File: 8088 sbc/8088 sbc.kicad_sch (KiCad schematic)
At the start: 15 parts, among them U1 8088, U2 74HC573, U3 74HC573, U4 28C256, U5 74HCT00, U6 HM628512, U7 74LS08

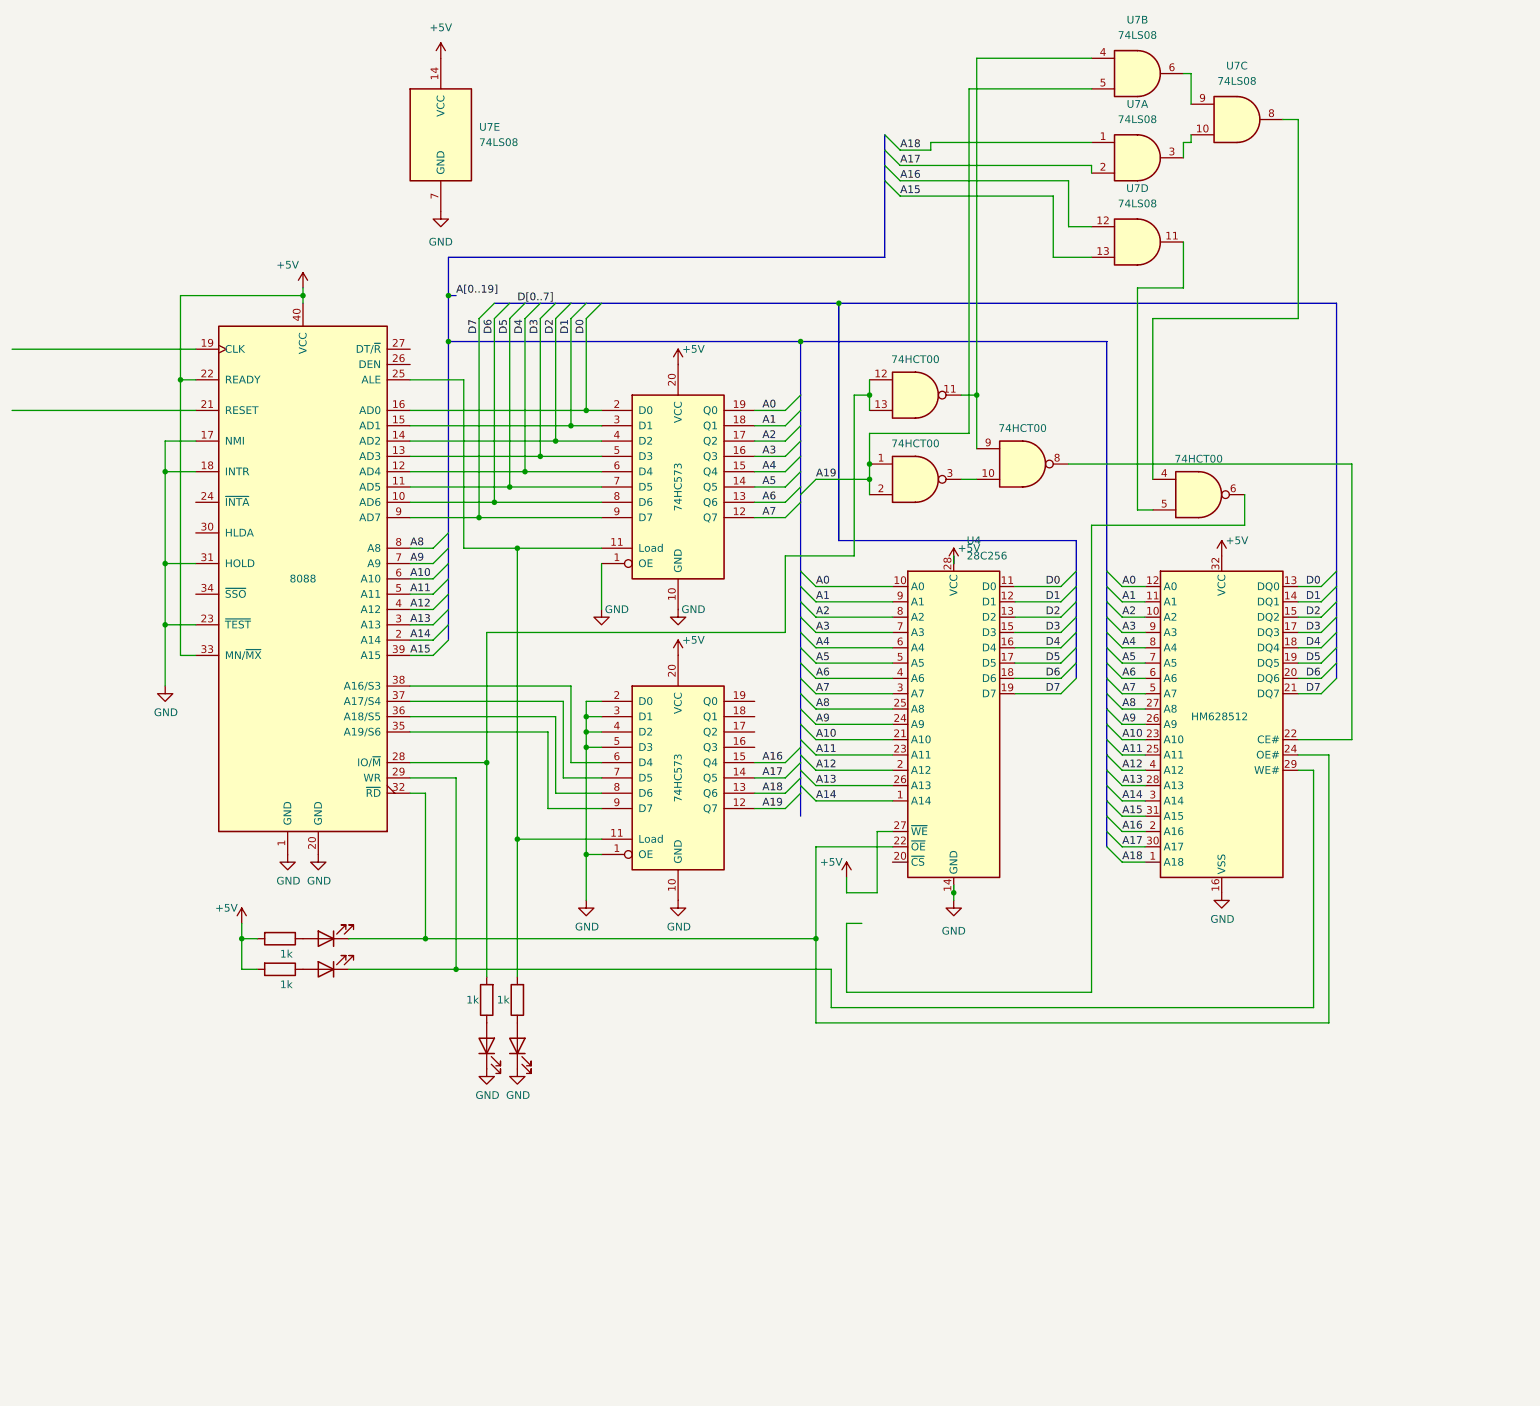
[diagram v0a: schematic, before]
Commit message: e
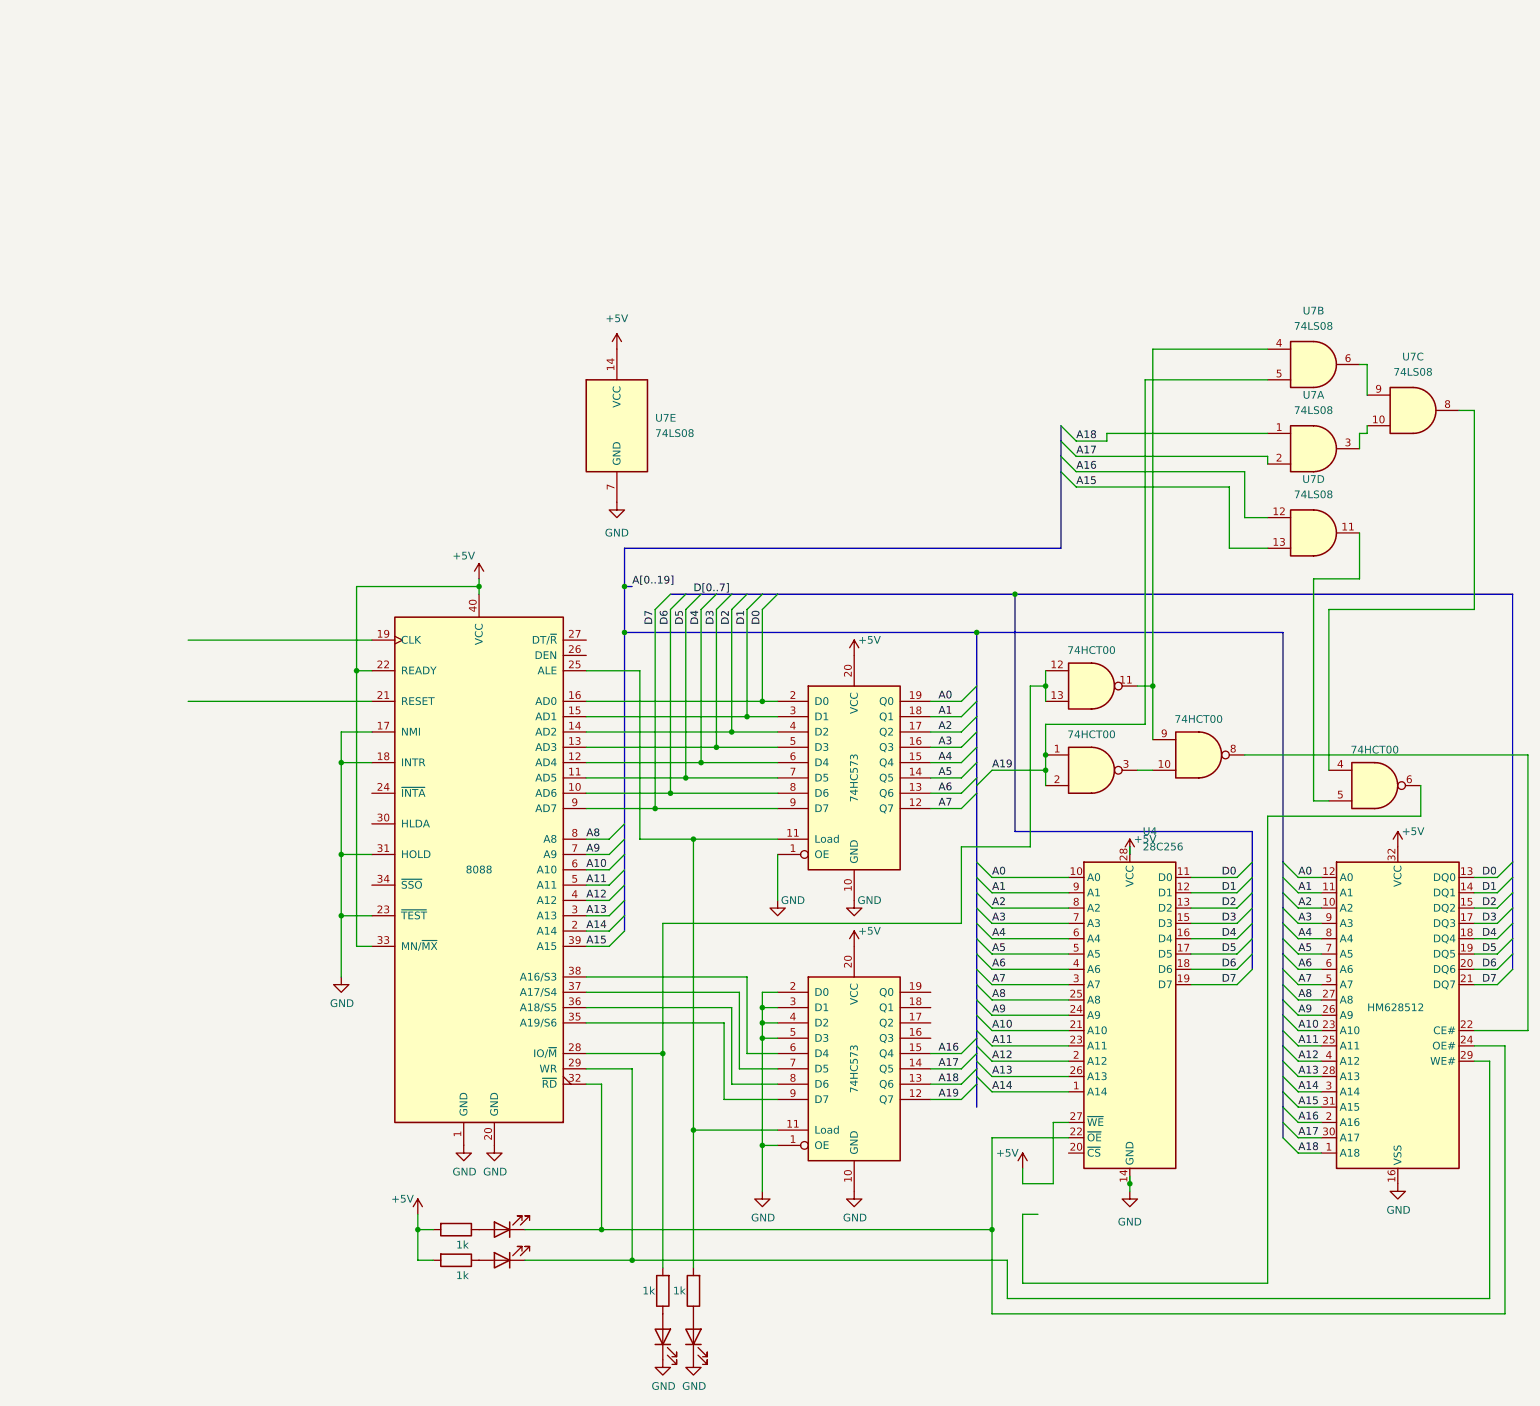
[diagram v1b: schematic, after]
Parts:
- gave numbers to parts that had none: 8
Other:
- moved on the sheet: U4, U7A, U7B, U7C, U7D, U7E
